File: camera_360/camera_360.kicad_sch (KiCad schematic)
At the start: 34 parts, among them J1 USB_C_Receptacle_USB2.0_14P, J2 usb_cam1, J3 usb_cam2, J4 usb_cam3, J5 usb_in, U1 CH334R, U2 USBLC6-2SC6, U3 USBLC6-2SC6, Y1 12Mhz

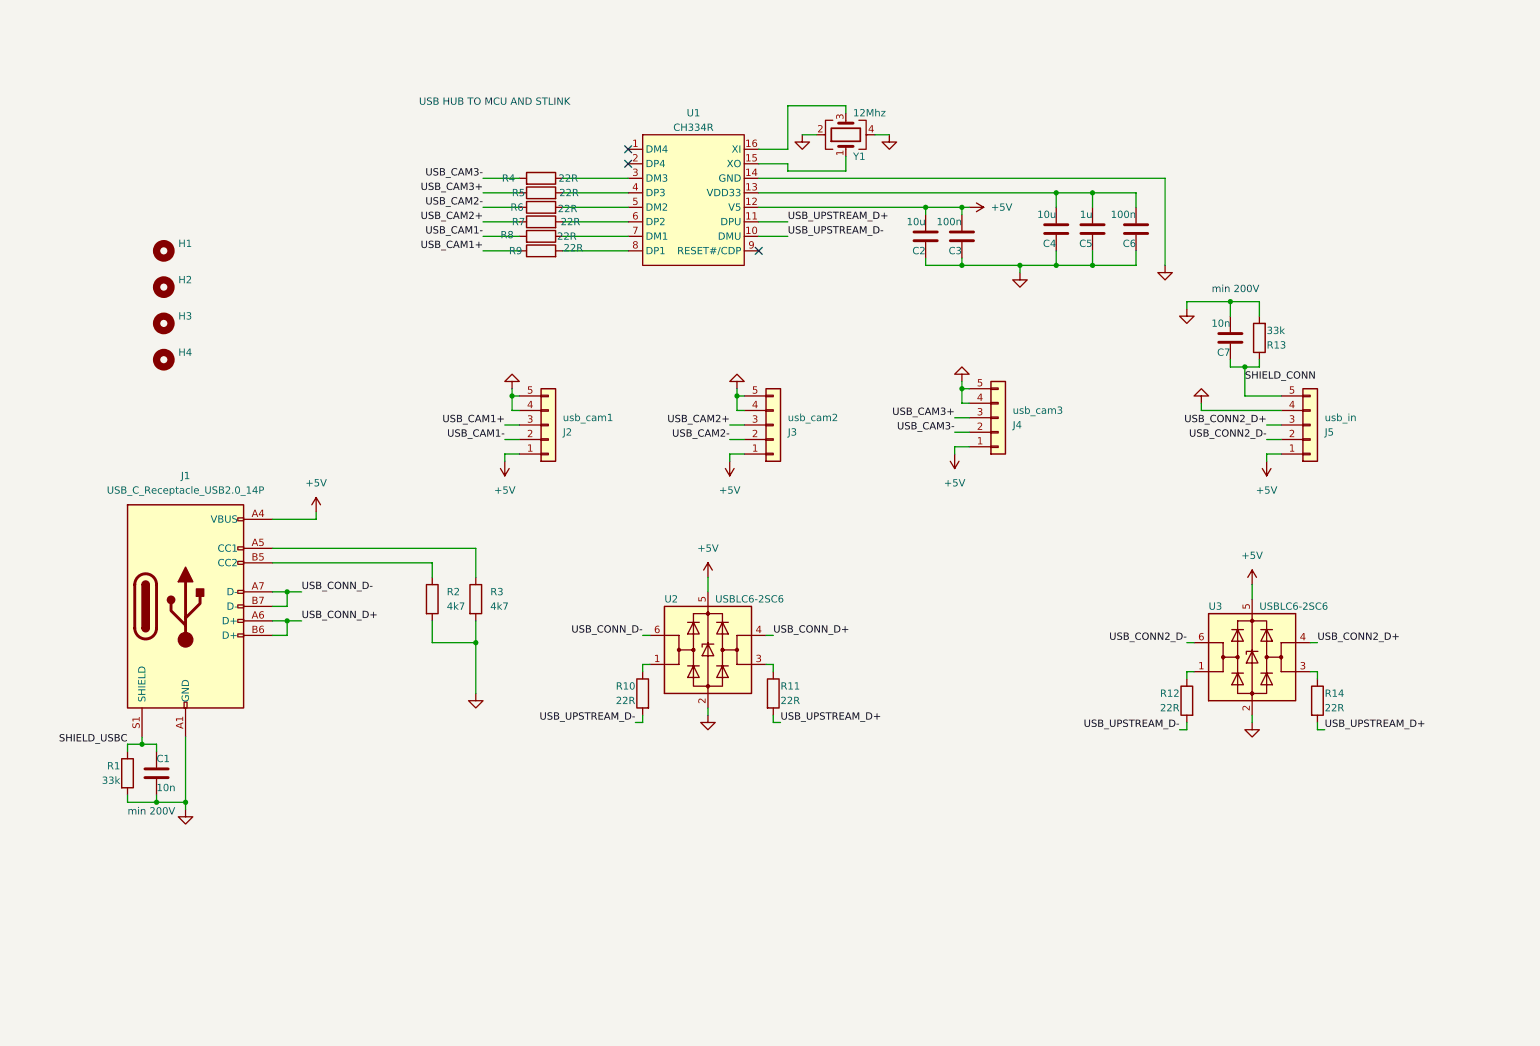
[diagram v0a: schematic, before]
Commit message: final revA
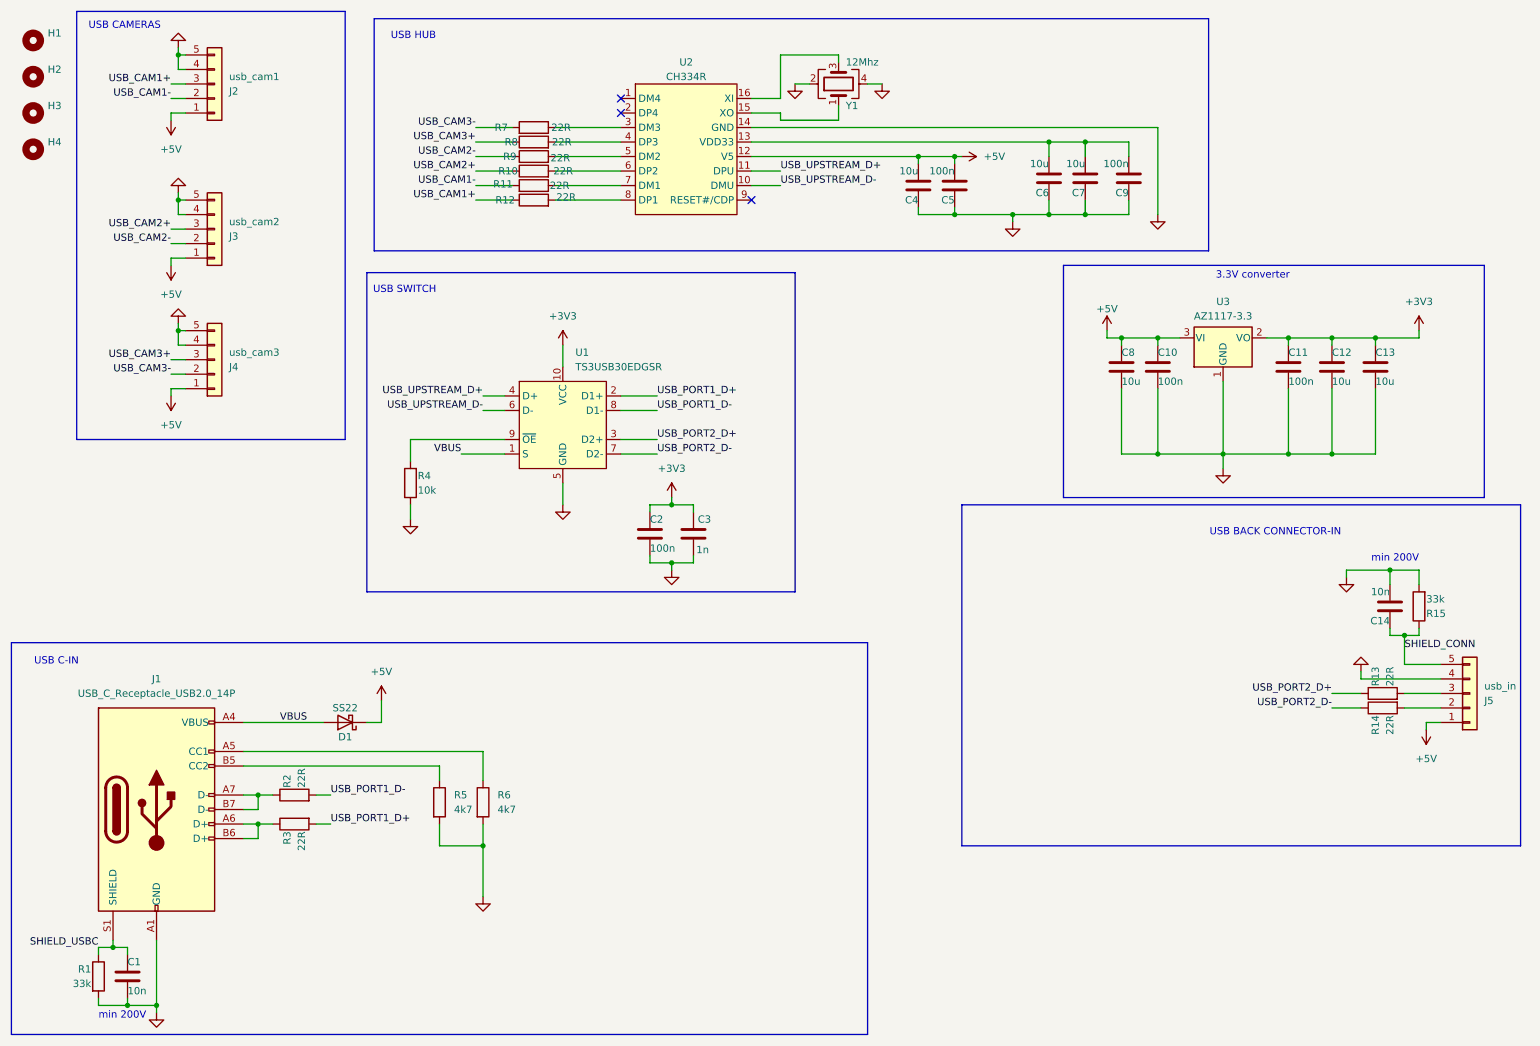
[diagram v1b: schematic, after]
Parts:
- removed R10, R11, R12: 22R, Resistor_SMD:R_0402_1005Metric, symbol Device:R
- removed U2, U3: USBLC6-2SC6, Package_TO_SOT_SMD:SOT-23-6, symbol Power_Protection:USBLC6-2SC6
- added C10, C11: 100n, Capacitor_SMD:C_0603_1608Metric, symbol Device:C
- added C12, C13, C8: 10u, Capacitor_SMD:C_0805_2012Metric, symbol Device:C
- added C2: 100n, Capacitor_SMD:C_0402_1005Metric, symbol Device:C
- added C3: 1n, Capacitor_SMD:C_0402_1005Metric, symbol Device:C
- added D1: SS22, Diode_SMD:D_SMA, symbol Device:D_Schottky
- added R13, R2, R3: 22R, Resistor_SMD:R_0402_1005Metric, symbol Device:R
- added R4: 10k, Resistor_SMD:R_0402_1005Metric, symbol Device:R
- added U1: TS3USB30EDGSR, Package_SO:VSSOP-10_3x3mm_P0.5mm, symbol Interface_USB:TS3USB30EDGSR
- added U3: AZ1117-3.3, Package_TO_SOT_SMD:SOT-223-3_TabPin2, symbol Regulator_Linear:AMS1117-3.3
- C7: renamed from C5; value 1u -> 10u; footprint Capacitor_SMD:C_0603_1608Metric -> Capacitor_SMD:C_0805_2012Metric
- R5: renamed from R2; footprint (none) -> Resistor_SMD:R_0402_1005Metric
- R6: renamed from R3; footprint (none) -> Resistor_SMD:R_0402_1005Metric
- renumbered C7 to C14, C2 to C4, C3 to C5, C4 to C6, C6 to C9, R7 to R10, R8 to R11, R9 to R12, R13 to R15, R4 to R7, R5 to R8, R6 to R9, U1 to U2
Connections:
- net +5V: now also C10.1, C8.1, D1.1 (K), U3.3 (VI); no longer J1.A4 (VBUS), J1.A9 (VBUS), J1.B4 (VBUS), J1.B9 (VBUS)
- net GND: now also C10.2, C11.2, C12.2, C13.2, C2.2, C3.2, C8.2, R4.1, U1.5 (GND), U3.1 (GND)
- net USB_UPSTREAM_D+: now also U1.4 (D+); no longer R14.2
- net USB_UPSTREAM_D-: now also U1.6 (D-)
- net USB_PORT2_D-: now reaches R14.1
- net USB_PORT2_D-: now also U1.7 (D2-)
- net USB_CONN2_D+: no longer names the net of J5.3 (Pin_3)
- net USB_CONN2_D+: now also R13.2
- net USB_CONN2_D-: no longer names the net of J5.2 (Pin_2)
- net USB_CONN2_D-: now also R14.2
- net USB_CONN_D+: no longer names the net of J1.A6 (D+), J1.B6 (D+)
- net USB_CONN_D+: now also R3.1
- net USB_CONN_D-: no longer names the net of J1.A7 (D-), J1.B7 (D-)
- net USB_CONN_D-: now also R2.1
- new net: R4.2, U1.9 (~{OE})
- new net +3V3: C11.1, C12.1, C13.1, C2.1, C3.1, U1.10 (VCC), U3.2 (VO)
- new net USB_PORT1_D+: R3.2, U1.2 (D1+)
- new net USB_PORT1_D-: R2.2, U1.8 (D1-)
- new net USB_PORT2_D+: R13.1, U1.3 (D2+)
- new net VBUS: D1.2 (A), J1.A4 (VBUS), J1.A9 (VBUS), J1.B4 (VBUS), J1.B9 (VBUS), U1.1 (S)
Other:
- note added: "3.3V converter"
- note added: "USB BACK CONNECTOR-IN"
- note added: "USB C-IN"
- note added: "USB CAMERAS"
- note added: "USB HUB"
- note added: "USB SWITCH"
- note removed: "USB HUB TO MCU AND STLINK"
- moved on the sheet: C1, C14, C4, C5, C6, C7, C9, H1, H2, H3, H4, J1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

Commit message: chaged uusb connectro to jst mx1.25
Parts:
- J2, J3, J4: footprint Connector_PinHeader_1.00mm:PinHeader_1x05_P1.00mm_Vertical -> Connector_JST:JST_GH_BM05B-GHS-TBT_1x05-1MP_P1.25mm_Vertical
- J5: footprint Connector_JST:JST_SH_BM05B-SRSS-TB_1x05-1MP_P1.00mm_Vertical -> Connector_JST:JST_GH_BM05B-GHS-TBT_1x05-1MP_P1.25mm_Vertical
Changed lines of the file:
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@@
 			)
 		)
-		(property "Footprint" "Connector_JST:JST_SH_BM05B-SRSS-TB_1x05-1MP_P1.00mm_Vertical"
+		(property "Footprint" "Connector_JST:JST_GH_BM05B-GHS-TBT_1x05-1MP_P1.25mm_Vertical"
 			(at 270.51 135.89 0)
 			(effects
@@
 			)
 		)
-		(property "Footprint" "Connector_PinHeader_1.00mm:PinHeader_1x05_P1.00mm_Vertical"
+		(property "Footprint" "Connector_JST:JST_GH_BM05B-GHS-TBT_1x05-1MP_P1.25mm_Vertical"
 			(at 50.8 77.47 0)
 			(effects
@@
 			)
 		)
-		(property "Footprint" "Connector_PinHeader_1.00mm:PinHeader_1x05_P1.00mm_Vertical"
+		(property "Footprint" "Connector_JST:JST_GH_BM05B-GHS-TBT_1x05-1MP_P1.25mm_Vertical"
 			(at 50.8 29.21 0)
 			(effects
@@
 			)
 		)
-		(property "Footprint" "Connector_PinHeader_1.00mm:PinHeader_1x05_P1.00mm_Vertical"
+		(property "Footprint" "Connector_JST:JST_GH_BM05B-GHS-TBT_1x05-1MP_P1.25mm_Vertical"
 			(at 50.8 54.61 0)
 			(effects
